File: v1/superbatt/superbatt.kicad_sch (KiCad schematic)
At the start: 14 parts, among them J1 Screw_Terminal_01x02, J2 Conn_01x02_Socket, J3 USB_B_Micro, J4 Screw_Terminal_01x02, J5 Conn_01x02_Socket

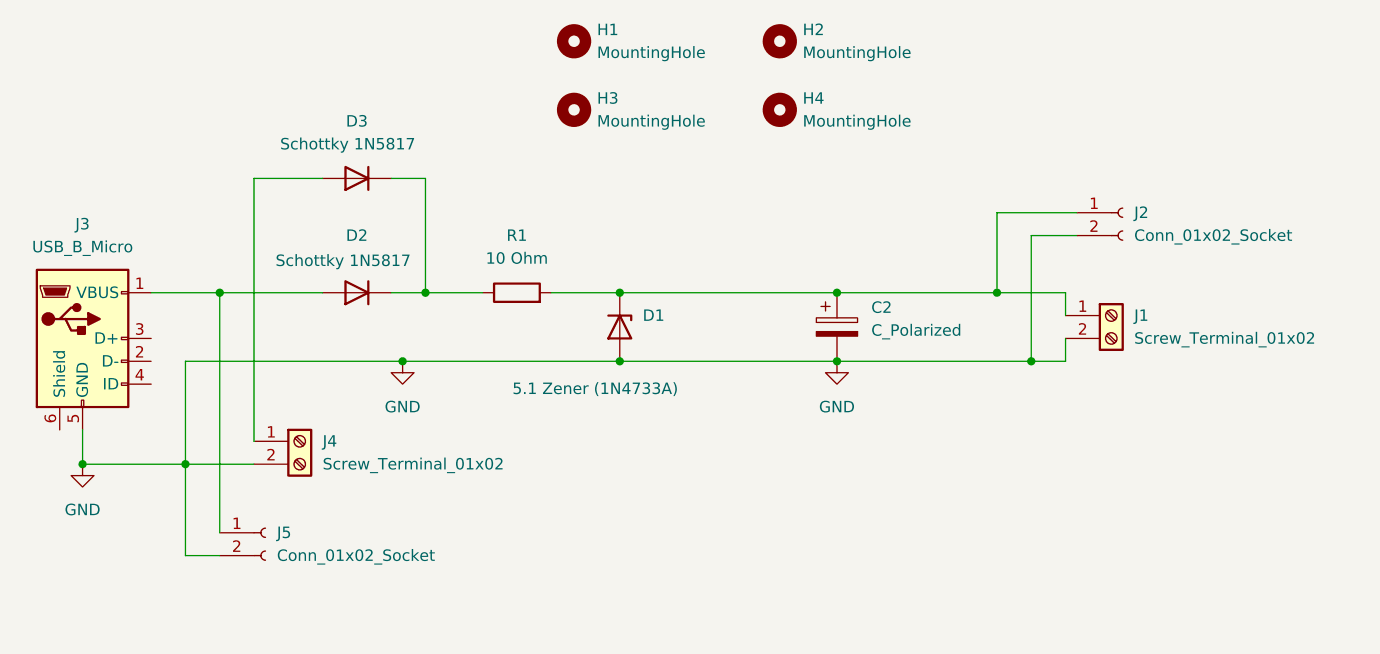
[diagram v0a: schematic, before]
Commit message: update
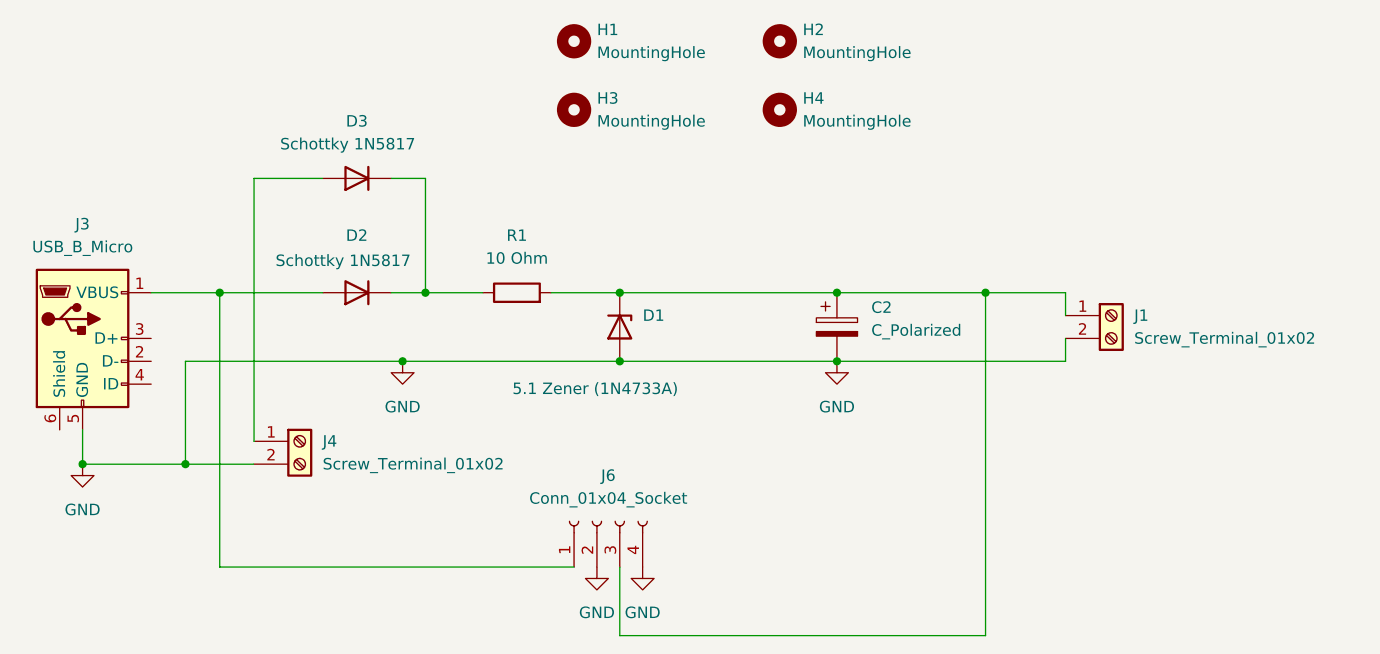
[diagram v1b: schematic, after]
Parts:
- removed J2, J5: Conn_01x02_Socket, Connector_PinHeader_2.54mm:PinHeader_1x02_P2.54mm_Vertical, symbol Connector:Conn_01x02_Socket
- added J6: Conn_01x04_Socket, Connector_PinSocket_2.54mm:PinSocket_1x04_P2.54mm_Vertical, symbol Connector:Conn_01x04_Socket
- C2: footprint Capacitor_THT:CP_Radial_D13.0mm_P5.00mm -> superbatt:CP_Radial_D22.0mm_P5.00mm_SnapIn
- R1: footprint Resistor_THT:R_Axial_DIN0309_L9.0mm_D3.2mm_P12.70mm_Horizontal -> Resistor_THT:R_Axial_DIN0207_L6.3mm_D2.5mm_P10.16mm_Horizontal
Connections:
- net GND: now also J6.2 (Pin_2), J6.4 (Pin_4)
- net at D2.2 (A), J3.1 (VBUS): now also J6.1 (Pin_1)
- net at C2.1, D1.1 (K), J1.1 (Pin_1)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: now also J6.3 (Pin_3)
